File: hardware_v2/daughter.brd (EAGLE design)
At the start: 78.5 x 56 mm, 32 parts, among them IC1 LM1117IMPX-3.3, K1 PIN20X2, Q1 8.00MHz, U2 MCP2551-I/SN, U4 TPS27081A, X1 MABC48B2

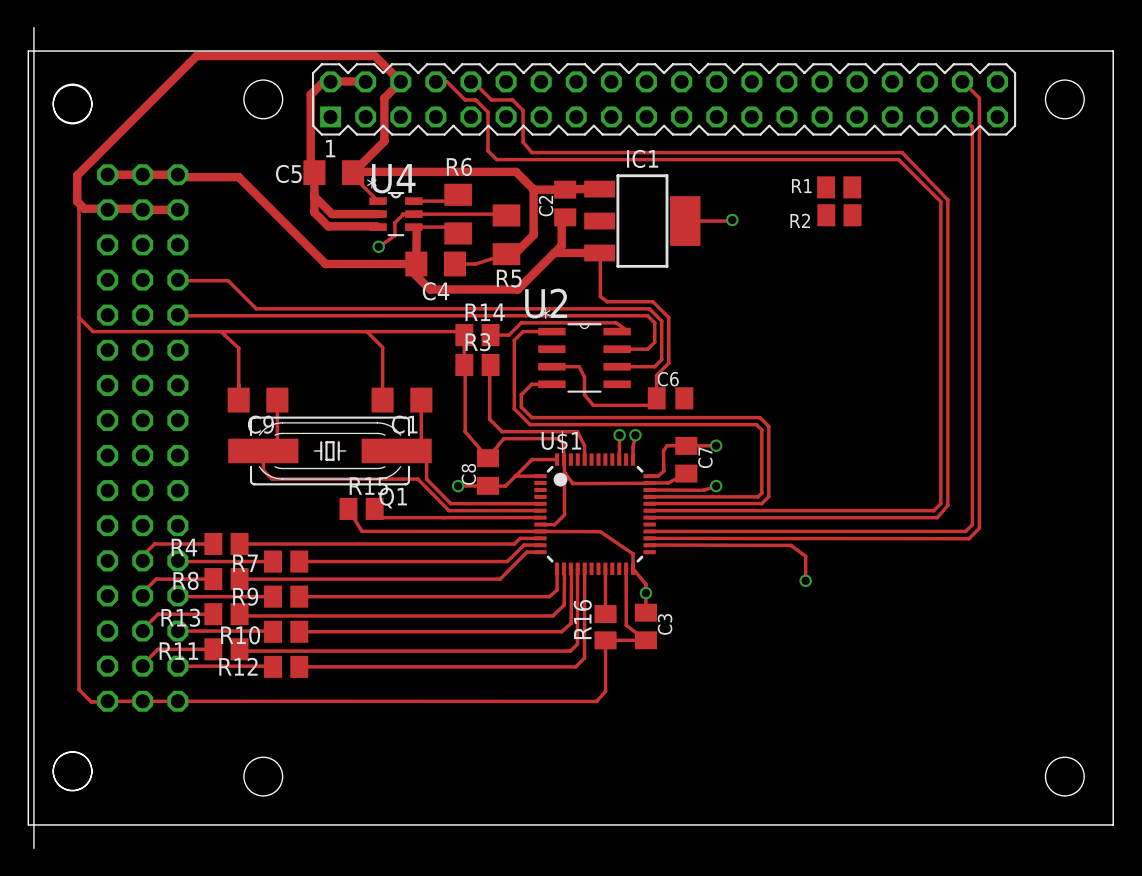
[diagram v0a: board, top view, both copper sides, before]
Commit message: hardware_v2: iteration after prelim board milling
Try the 8mhz and 32khz oscillators off-baord, e.g.
shared across the bus.  Experiment with drivers,
conditioning, termination later.

BOOT0 and BOOT1 are tied to ground via 10K resistors.
NRST is tied high via 10K resistor.

Wire the two STM32 slave I2C busses: pi ID EEPROM
emulation and general pi signaling.

IDENTIFY, LCAN-ACT, ALIVE, and +5V power LEDs
are populated but not connected yet.  Possibly the
active LEDs will be folded in with SPI-driven
MAX7212 LED array.
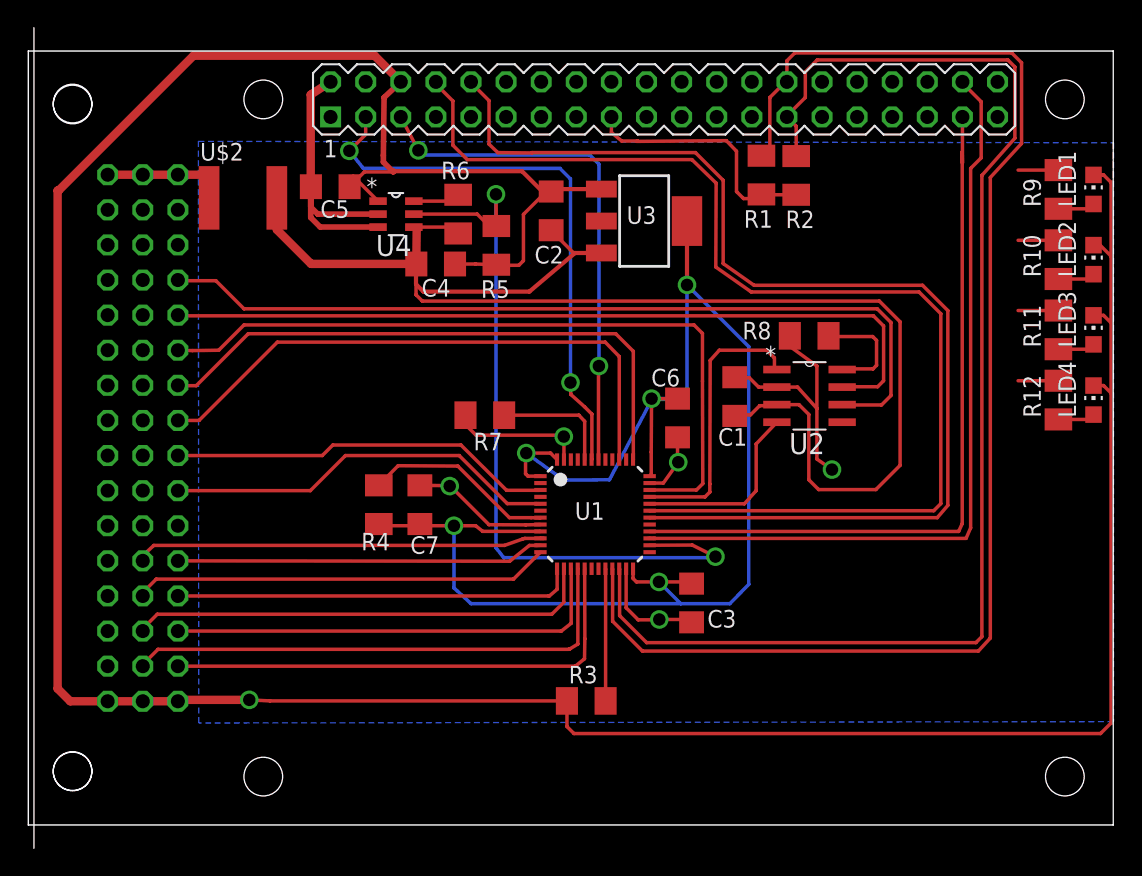
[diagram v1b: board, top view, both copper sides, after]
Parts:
- removed C8: 100nF, resistor:C0805K
- removed C9: 22pF, resistor:C1206
- removed IC1: LM1117IMPX-3.3, lm1117:SOT223
- removed Q1: 8.00MHz, crystal:SM49
- removed R13, R15, R16: 10K, resistor:M0805
- removed R14: 10k, resistor:M0805
- added LED1, LED2, LED3, LED4: (no value), led:CHIP-LED0805
- added U$2: MF-SMDF050, fuse:MF-SMDF050
- added U3: LM1117IMPX-3.3, lm1117:SOT223
- C1: value 22pF -> 100nF
- C2: value 10uF -> 100nF; device resistor:C0805K -> resistor:C1206
- C3, C6, C7: device resistor:C0805K -> resistor:C1206
- R1, R2: value 3k9 -> 3K9; device resistor:M0805 -> resistor:M1206
- R10, R11, R12: value 10K -> 220; device resistor:M0805 -> resistor:M1206
- R3, R4, R7, R8: device resistor:M0805 -> resistor:M1206
- R9: value 10K -> 330; device resistor:M0805 -> resistor:M1206
- moved R11 64.5 mm to (106.9, 39.6), turned to 90 degrees
- moved R9 63.2 mm to (106.9, 49.8), turned to 90 degrees
- moved R10 62.0 mm to (106.9, 44.7), turned to 90 degrees
- moved R12 59.1 mm to (106.9, 34.5), turned to 90 degrees
- moved R8 45.7 mm to (88.9, 39.2), turned to 0 degrees
- moved R3 25.6 mm to (72.8, 12.8)
- moved C1 24.1 mm to (83.5, 34.8), turned to 90 degrees
- moved C7 19.6 mm to (60.7, 27.0), turned to 90 degrees
- moved R7 17.9 mm to (65.4, 33.5)
- moved U2 16.5 mm to (88.9, 34.8)
- moved R4 11.4 mm to (57.8, 27.0), turned to 270 degrees
- moved R1 5.70 mm to (85.4, 50.8), turned to 270 degrees
- moved R2 4.25 mm to (88.0, 50.8), turned to 270 degrees
- moved C3 3.71 mm to (80.4, 19.9)
- moved C6 1.51 mm to (79.4, 33.2), turned to 270 degrees
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- renumbered U$1 to U1
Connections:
- removed net N$10: R12.1, U1.17
- removed net N$11: R16.2, U1.20
- removed net N$12: U2.2
- removed net N$2: R4.1, U1.10
- removed net XTALA: C1.1, Q1.1, U1.5
- removed net XTALB: C9.1, Q1.2, U1.6
- removed net XTALC: U1.3
- removed net XTALD: U1.4
- new net ALIVE: R12.2, U1.25
- new net IDENTIFY: R11.2, U1.46
- new net LCAN-ACT: R10.2, U1.41
- new net OSC-HSE: U1.5, X1.C10
- new net OSC-LSE: U1.3, X1.C9
- new net SCL: K1.5, U1.42
- new net SDA: K1.3, U1.43
- net +5V: now also R9.2
- net BUS5V: now also C1.1, U$2.2, U3.3; no longer C6.1, IC1.3, X1.A1, X1.B1, X1.C1
- net GND: now also LED1.C, LED2.C, LED3.C, LED4.C, R7.2, R8.1, U2.2, U3.1; no longer C8.2, C9.2, IC1.1, R14.1, R16.1, X1.A2, X1.B2, X1.C2
- net ID-SC: now also R1.1, U1.21; no longer R2.1
- net ID-SD: now also R2.1, U1.22; no longer R1.1
- net MOD-A0: now also U1.14; no longer R13.2
- net MOD-A1: now also U1.15; no longer R10.2
- net MOD-A2: now also U1.16; no longer R11.2
- net MOD-A3: now also U1.17; no longer R12.2
- net N$16: now also R8.2; no longer R14.2
- net N$3: now also R7.1; no longer R3.2
- net N$4: now also U$2.1, X1.A1, X1.B1, X1.C1; no longer R7.1, U1.11
- net N$5: now also LED4.A, R12.1; no longer R8.1, U1.12
- net N$6: now also R3.2, U1.20; no longer R9.1, U1.13
- net N$7: now also LED3.A, R11.1; no longer R13.1, U1.14
- net N$8: now also LED2.A; no longer U1.15
- net N$9: now also LED1.A, R9.1; no longer R11.1, U1.16
- net NODE-A0: now also U1.10; no longer R4.2
- net NODE-A1: now also U1.11; no longer R7.2
- net NODE-A2: now also U1.12; no longer R8.2
- net NODE-A3: now also U1.13; no longer R9.2
- net NRST: now also R4.1; no longer R15.2
- net STBY3V3: now also C6.1, R4.2, U3.2, U3.TAB; no longer C8.1, IC1.2, IC1.TAB, R15.1
- net SWCLK: now also X1.C7; no longer X1.A4
- net SWDIO: now also X1.C6; no longer X1.A3
- net SWO: now also X1.C8; no longer X1.A5
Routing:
- net ID-SC: track 0.00 -> 100.2 mm
- net ID-SD: track 0.00 -> 95.4 mm
- net STBY3V3: track 46.5 -> 112.4 mm, vias 4 -> 5
- net SWDIO: track 4.86 -> 53.9 mm, vias 1 -> 0
- net GND: track 237.5 -> 281.5 mm, vias 0 -> 6
- net SWCLK: track 1.78 -> 42.9 mm, vias 1 -> 0
- net SDA: track 0.00 -> 40.8 mm, vias 0 -> 2
- net SWO: track 1.77 -> 42.2 mm, vias 1 -> 0
- net SCL: track 0.00 -> 37.6 mm, vias 0 -> 2
- net MOD-A2: track 5.68 -> 37.6 mm
- net BUS5V: track 73.4 -> 105.2 mm
- net PWR-ON: track 24.1 -> 54.8 mm
- net MOD-A3: track 6.90 -> 36.1 mm
- net OSC-HSE: track 0.00 -> 28.7 mm
- net MOD-A0: track 5.68 -> 33.9 mm
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- added copper zone on layer 16, net GND
